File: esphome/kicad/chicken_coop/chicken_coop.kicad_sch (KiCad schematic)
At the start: 3 parts, among them J1 Conn_01x04_Pin, U1 ESP32-CAM

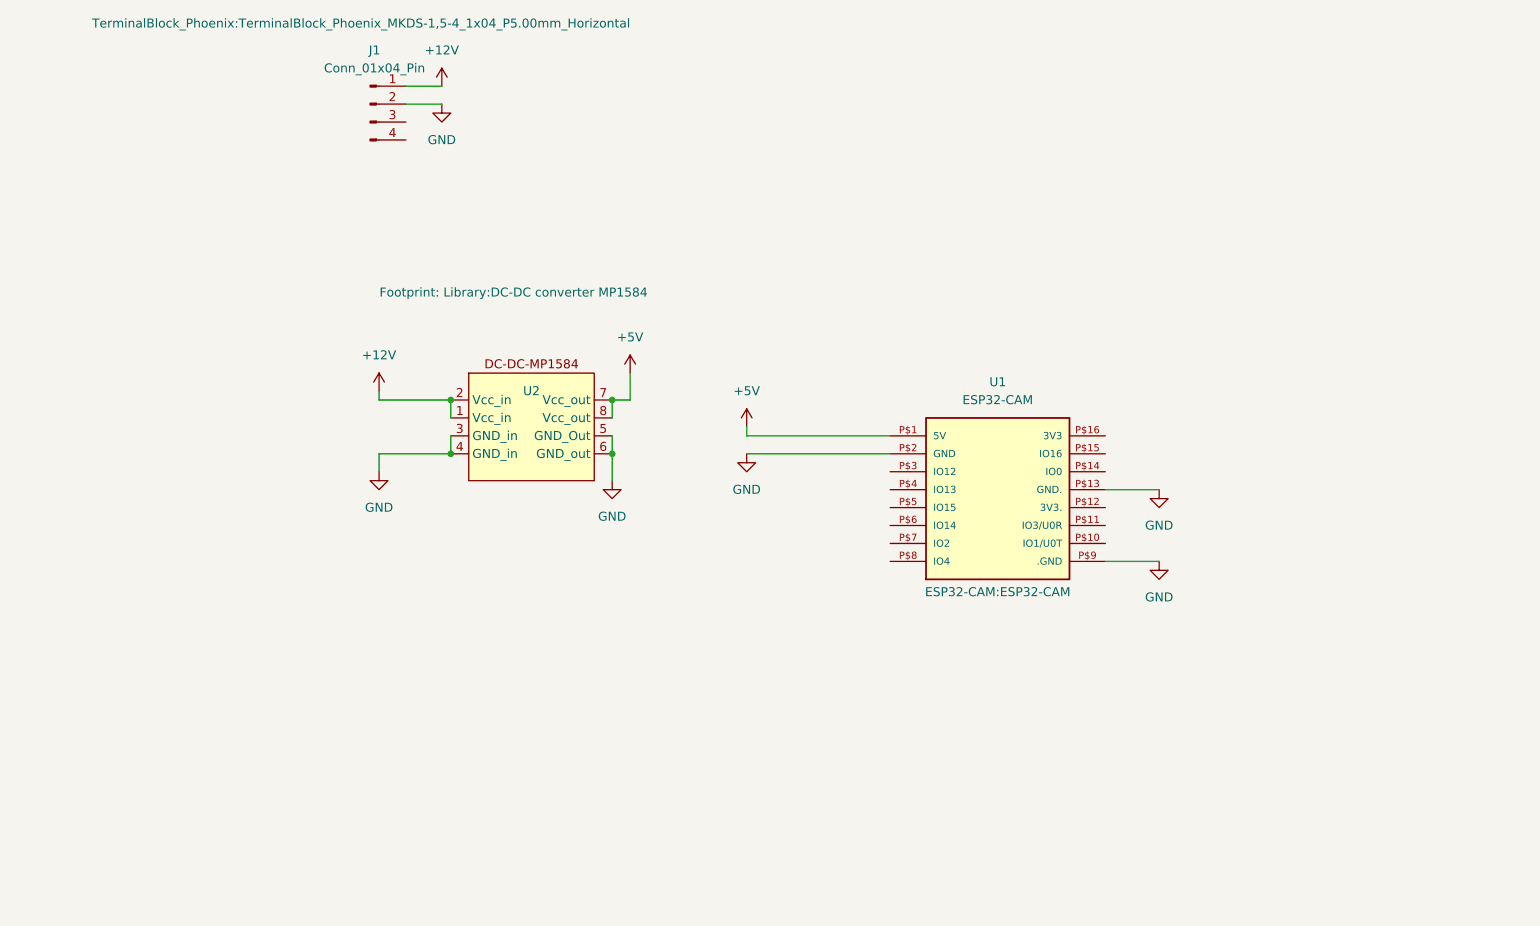
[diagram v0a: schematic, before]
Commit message: sync
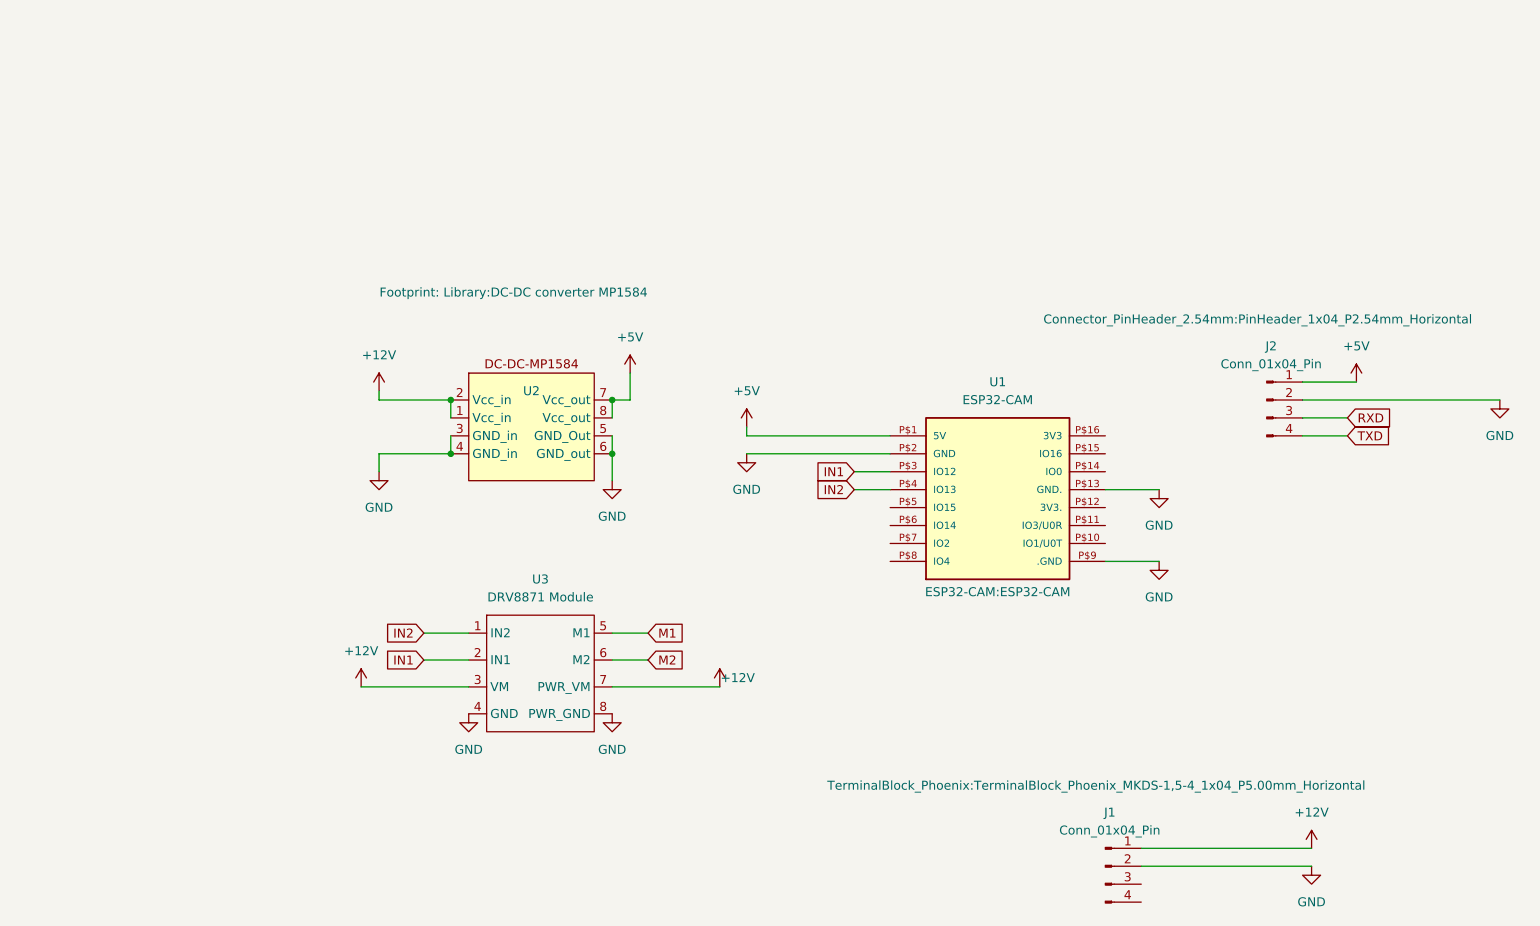
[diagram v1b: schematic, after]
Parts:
- added J2: Conn_01x04_Pin, Connector_PinHeader_2.54mm:PinHeader_1x04_P2.54mm_Horizontal, symbol Connector:Conn_01x04_Pin
- added U3: DRV8871 Module, symbol custom:DRV8871_Module
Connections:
- net +12V: now also U3.3 (VM), U3.7 (PWR_VM)
- net +5V: now also J2.1 (Pin_1)
- net GND: now also J2.2 (Pin_2), U3.4 (GND), U3.8 (PWR_GND)
- net IN1: now reaches U1.P$3 (IO12)
- net IN1: now also U3.2 (IN1)
- net IN2: now reaches U1.P$4 (IO13)
- net IN2: now also U3.1 (IN2)
- new net M1: U3.5 (M1)
- new net M2: U3.6 (M2)
- new net RXD: J2.3 (Pin_3)
- new net TXD: J2.4 (Pin_4)
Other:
- moved on the sheet: J1
